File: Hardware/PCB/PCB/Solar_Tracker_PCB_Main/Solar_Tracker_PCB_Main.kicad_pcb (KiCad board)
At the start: 4 copper layers, 95.4 x 96.8 mm, 59 parts, among them IC1 ESP32-S3-WROOM-1-N4R8, IC2 TPS54302DDCT, IC3 BNO085, IC4 PCF2131TFY, IC5 LM1117MPX-3.3_NOPB, J1 1729076, J2 USB4940-00-A, J3 1729076, J4 1977223-1, J5 1977223-1, J6 1729076, J7 TB002-500-02BE, Y1 32.768kHz

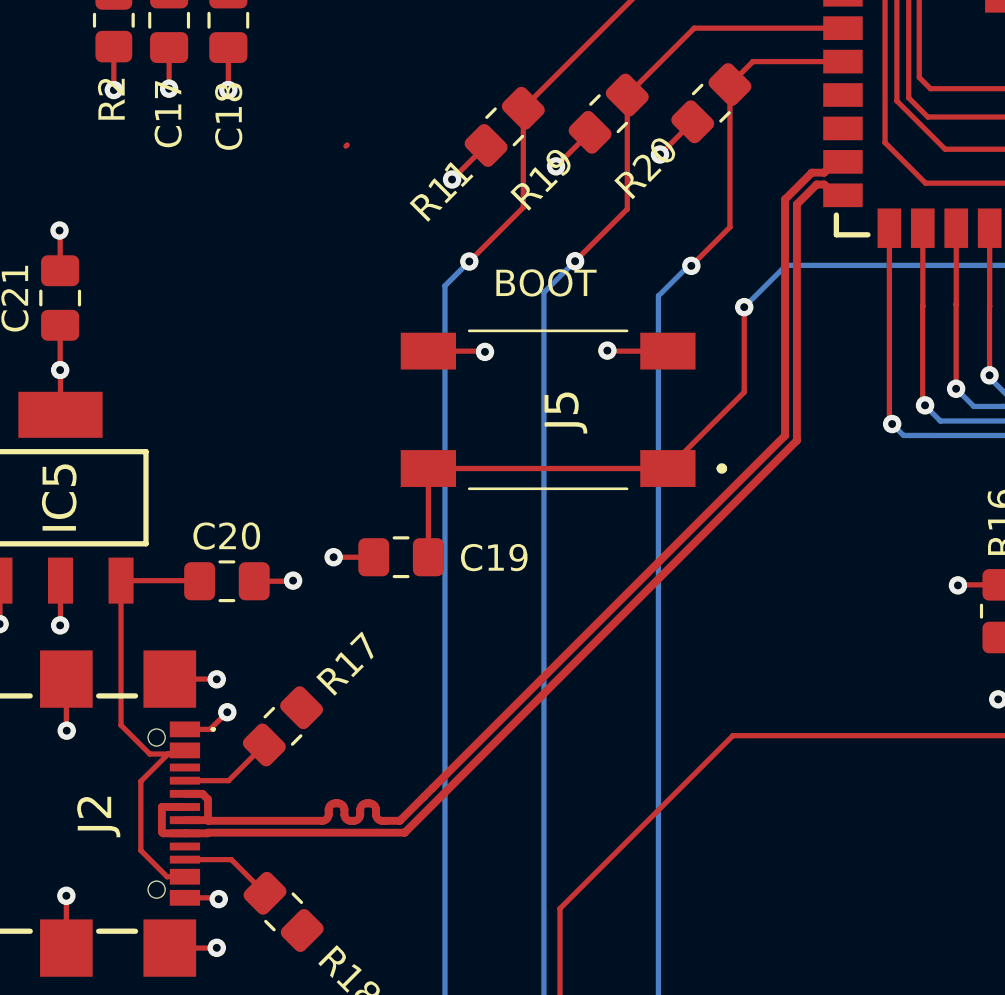
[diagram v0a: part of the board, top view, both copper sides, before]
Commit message: Par deferencial
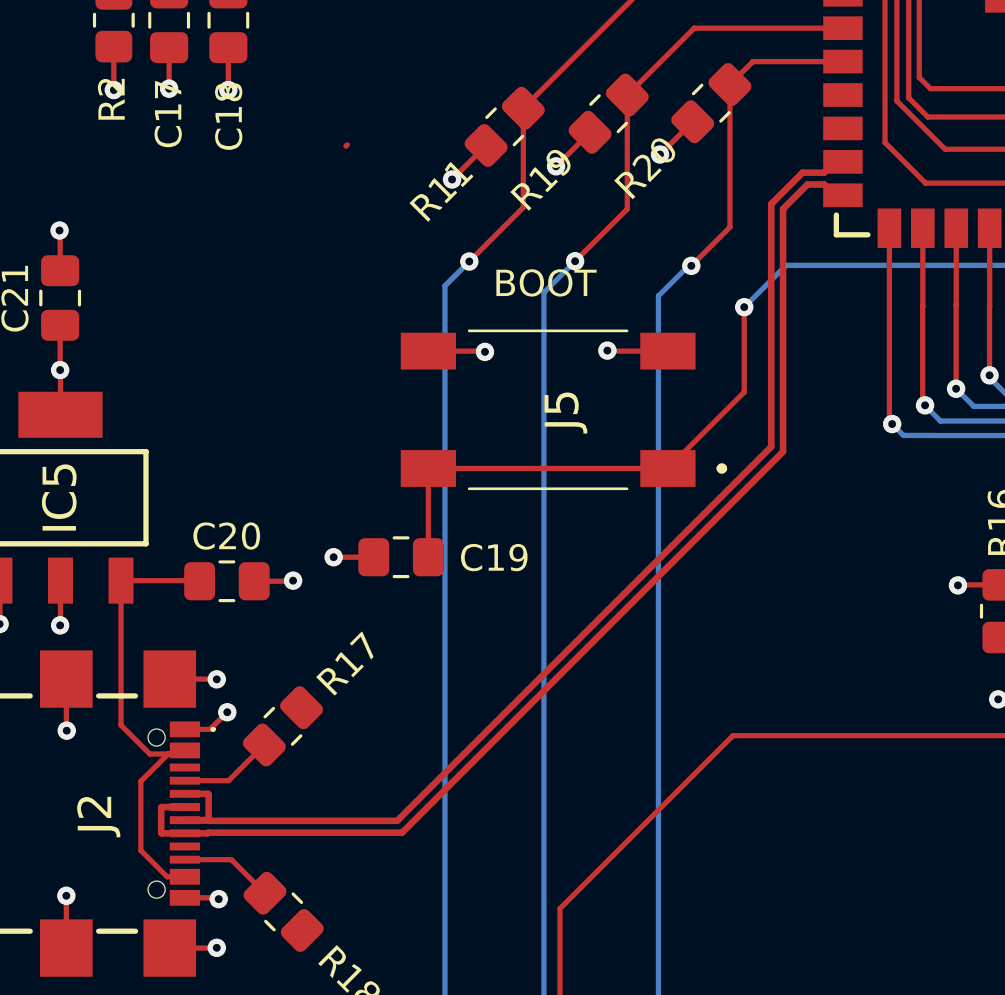
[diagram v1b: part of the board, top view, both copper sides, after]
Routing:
- net D-: track 44.1 -> 43.6 mm
